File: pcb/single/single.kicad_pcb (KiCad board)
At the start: 2 copper layers, 95 x 130 mm, 31 parts, among them J1 USB_A, J10 USB_A, J2 Barrel_Jack_Switch_DC10B, J3 Barrel_Jack_Switch_DC10B, J4 Barrel_Jack_Switch_DC10B, J5 Barrel_Jack_Switch_DC10B, J6 Barrel_Jack_Switch_DC10B, J7 USB_A, J8 USB_A, J9 USB_A, U1_12V1 i6A4W010A033V-001-R, U1_5V1 i6A4W010A033V-001-R

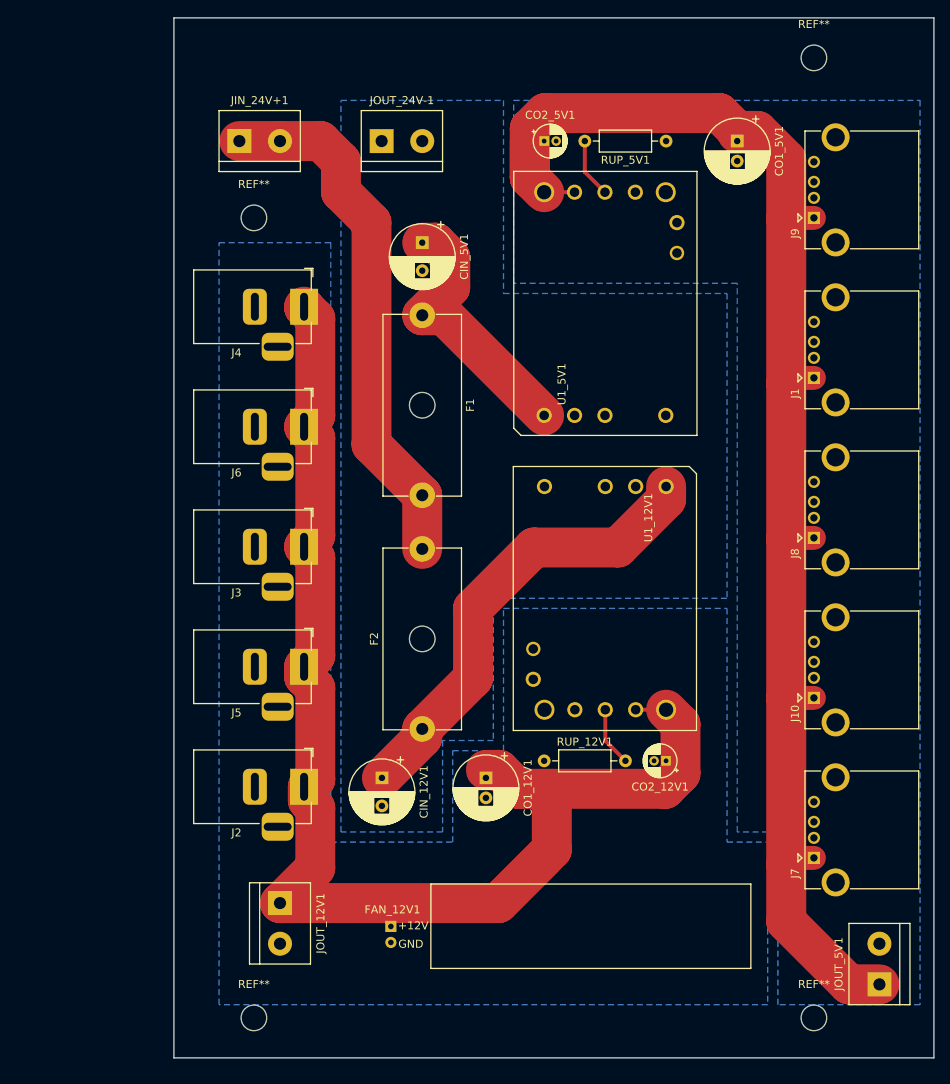
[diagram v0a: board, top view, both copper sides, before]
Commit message: As ordered
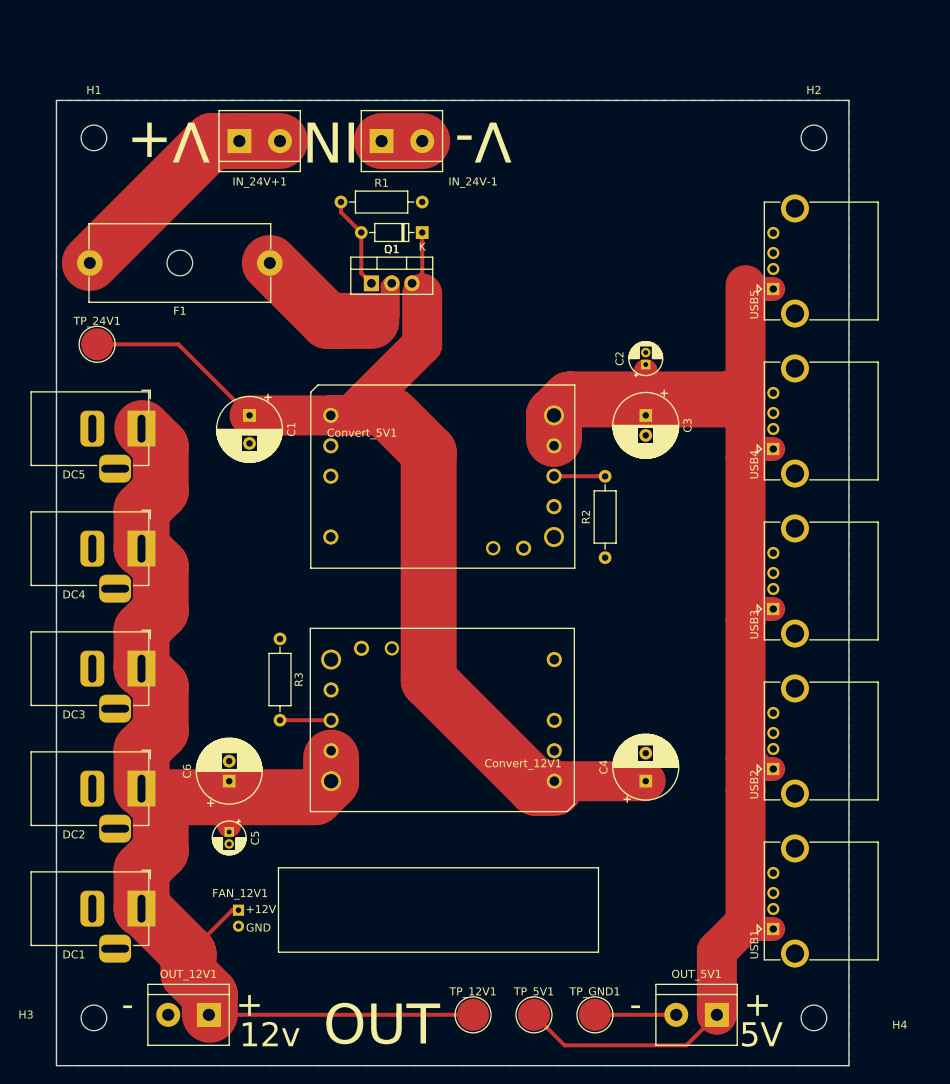
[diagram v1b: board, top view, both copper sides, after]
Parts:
- removed F2: Fuse, box_power:Fuseholder_Cylinder-5x20mm_646_series_22.6_1.5
- removed REF** (x4): MountingHole_3.2mm_M3, MountingHole:MountingHole_3.2mm_M3
- added D1: Zener_18V, Diode_THT:D_DO-35_SOD27_P7.62mm_Horizontal, F.Cu at (66.0, 36.8)
- added H1: MountingHole, MountingHole:MountingHole_3.2mm_M3, F.Cu at (25.0, 25.0)
- added H2: MountingHole, MountingHole:MountingHole_3.2mm_M3, F.Cu at (115.0, 25.0)
- added H3: MountingHole, MountingHole:MountingHole_3.2mm_M3, F.Cu at (25.0, 135.0)
- added H4: MountingHole, MountingHole:MountingHole_3.2mm_M3, F.Cu at (115.0, 135.0)
- added Q1: Q_PMOS_GDS, Package_TO_SOT_THT:TO-220-3_Vertical, F.Cu at (59.7, 43.2)
- added R1: 300R, Resistor_THT:R_Axial_DIN0207_L6.3mm_D2.5mm_P10.16mm_Horizontal, F.Cu at (55.9, 33.0)
- added TP_12V1: TestPoint, TestPoint:TestPoint_Pad_D4.0mm, F.Cu at (72.4, 134.6)
- added TP_24V1: TestPoint, TestPoint:TestPoint_Pad_D4.0mm, F.Cu at (25.4, 50.8)
- added TP_5V1: TestPoint, TestPoint:TestPoint_Pad_D4.0mm, F.Cu at (80.0, 134.6)
- added TP_GND1: TestPoint, TestPoint:TestPoint_Pad_D4.0mm, F.Cu at (87.6, 134.6)
- USB1: renamed from J1; value USB_A -> USB A
- USB2: renamed from J7; value USB_A -> USB A
- USB3: renamed from J8; value USB_A -> USB A
- USB4: renamed from J9; value USB_A -> USB A
- USB5: renamed from J10; value USB_A -> USB A
- moved USB1 69.1 mm to (109.9, 123.9)
- moved C5 55.3 mm to (41.9, 111.8), turned to 270 degrees
- moved R2 52.6 mm to (88.9, 77.5), turned to 90 degrees
- moved USB5 51.4 mm to (109.9, 43.9)
- moved DC3 49.6 mm to (30.9, 91.3)
- moved Convert_12V1 39.4 mm to (82.5, 105.4), turned to 180 degrees
- moved DC2 36.4 mm to (30.9, 106.3)
- moved R3 36.4 mm to (48.3, 87.6), turned to 270 degrees
- moved C3 36.1 mm to (94.0, 59.7)
- moved C4 33.0 mm to (94.0, 105.4), turned to 90 degrees
- moved C6 32.1 mm to (41.9, 105.4), turned to 90 degrees
- moved C2 30.7 mm to (94.0, 53.3), turned to 90 degrees
- moved C1 30.5 mm to (44.5, 59.7)
- moved USB4 29.3 mm to (109.9, 63.9)
- moved Convert_5V1 26.7 mm to (54.6, 59.7), turned to 0 degrees
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- renumbered CIN_5V1 to C1, CO2_5V1 to C2, CO1_5V1 to C3, CIN_12V1 to C4, CO2_12V1 to C5, CO1_12V1 to C6, U1_12V1 to Convert_12V1, U1_5V1 to Convert_5V1, J2 to DC1, J3 to DC2, J4 to DC3, J5 to DC4, J6 to DC5, JIN_24V+1 to IN_24V+1, JOUT_24V-1 to IN_24V-1, JOUT_12V1 to OUT_12V1, JOUT_5V1 to OUT_5V1, RUP_5V1 to R2, RUP_12V1 to R3
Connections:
- C1 pad 1: Net-(CIN_5V1-Pad1) -> 24V
- C2 pad 2: 5V_GND -> GND
- C3 pad 2: 5V_GND -> GND
- C4 pad 1: Net-(CIN_12V1-Pad1) -> 24V
- C5 pad 2: GND_12V -> GND
- C6 pad 2: GND_12V -> GND
- Convert_12V1 pad 1: Net-(CIN_12V1-Pad1) -> 24V
- Convert_12V1 pad 4: GND_12V -> GND
- Convert_5V1 pad 1: Net-(CIN_5V1-Pad1) -> 24V
- Convert_5V1 pad 4: 5V_GND -> GND
- DC1 pad 3: GND_12V -> GND
- DC2 pad 3: GND_12V -> GND
- DC3 pad 3: GND_12V -> GND
- DC4 pad 3: GND_12V -> GND
- DC5 pad 3: GND_12V -> GND
- F1 pad 1: Net-(CIN_5V1-Pad1) -> Net-(F1-Pad1)
- F1 pad 2: 24V -> Net-(F1-Pad2)
- FAN_12V1 pad 2: GND_12V -> GND
- IN_24V+1 pad 1: 24V -> Net-(F1-Pad2)
- IN_24V+1 pad 2: 24V -> Net-(F1-Pad2)
- OUT_12V1 pad 2: GND_12V -> GND
- OUT_5V1 pad 2: 5V_GND -> GND
- R2 pad 1: 5V_GND -> GND
- R3 pad 1: GND_12V -> GND
- USB1 pad 4: 5V_GND -> GND
- USB1 pad 5: 5V_GND -> GND
- USB2 pad 4: 5V_GND -> GND
- USB2 pad 5: 5V_GND -> GND
- USB3 pad 4: 5V_GND -> GND
- USB3 pad 5: 5V_GND -> GND
- USB4 pad 4: 5V_GND -> GND
- USB4 pad 5: 5V_GND -> GND
- USB5 pad 4: 5V_GND -> GND
- USB5 pad 5: 5V_GND -> GND
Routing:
- net 24V: track 66.4 -> 147.3 mm
- net Net-(CIN_12V1-Pad1): track 57.3 -> 0.00 mm
- net Net-(CIN_5V1-Pad1): track 33.4 -> 0.00 mm
- net Net-(F1-Pad2): track 0.00 -> 30.1 mm
- net 12V: track 187.3 -> 157.8 mm
- net Net-(F1-Pad1): track 0.00 -> 24.2 mm
- net GND: track 0.00 -> 15.2 mm
- net Net-(D1-Pad2): track 0.00 -> 11.7 mm
- net 5V: track 180.8 -> 172.3 mm
- net Net-(Convert_5V1-Pad6): track 7.43 -> 6.40 mm
- net Net-(Convert_12V1-Pad6): track 7.43 -> 6.40 mm
- removed copper zone on B.Cu, net 5V_GND
- removed copper zone on B.Cu, net GND_12V
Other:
- board size 95 x 130 mm -> 99.1 x 120.7 mm
- board text added: "+"
- board text added: "-"
- board text added: "12v"
- board text added: "5V"
- board text added: "IN"
- board text added: "OUT"
- board text added: "V+"
- board text added: "V-"
